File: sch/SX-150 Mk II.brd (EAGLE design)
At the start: 156.2 x 60.6 mm, 189 parts, among them IC1 LM358D, IC2 74HC02D, IC3 LM358D, IC4 LM386M-1, IC5 NJU7096, IC6 REG1117, J1 PJ301M, J2 Line In, Q1 2SC2712, Q10 2SC2712, Q11 2SA1162, Q12 2SC2712, Q13 2SC2712, Q14 2SC2712, Q15 2SC2712, Q16 2SC2712, Q17 2SC2712, Q18 2SC2712, Q19 2SC2712, Q2 2SC2712, Q20 2SC2712, Q21 2SC2712, Q22 2SC2712, Q23 2SC2712, Q24 2SA1162, Q25 2SC2712, Q26 2SC2712, Q27 2SC2712, Q28 2SC2712, Q3 2SC2712, Q4 2SC2712, Q5 2SC2712, Q6 2SC2712, Q7 2SC2712, Q8 2SA1162, Q9 2SC2712, SW1 SP3T, T1 50k, X2 Speaker Out

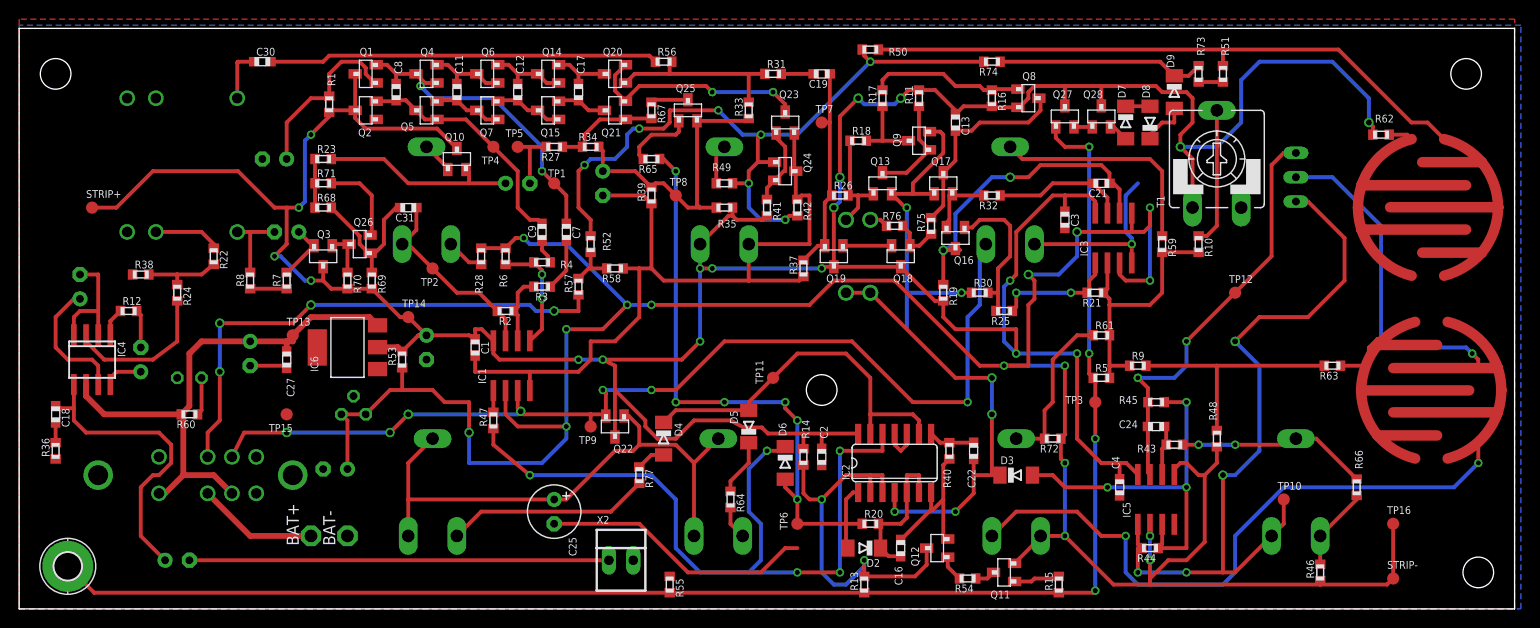
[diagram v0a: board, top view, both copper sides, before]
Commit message: Updating board layout and adding gerbers
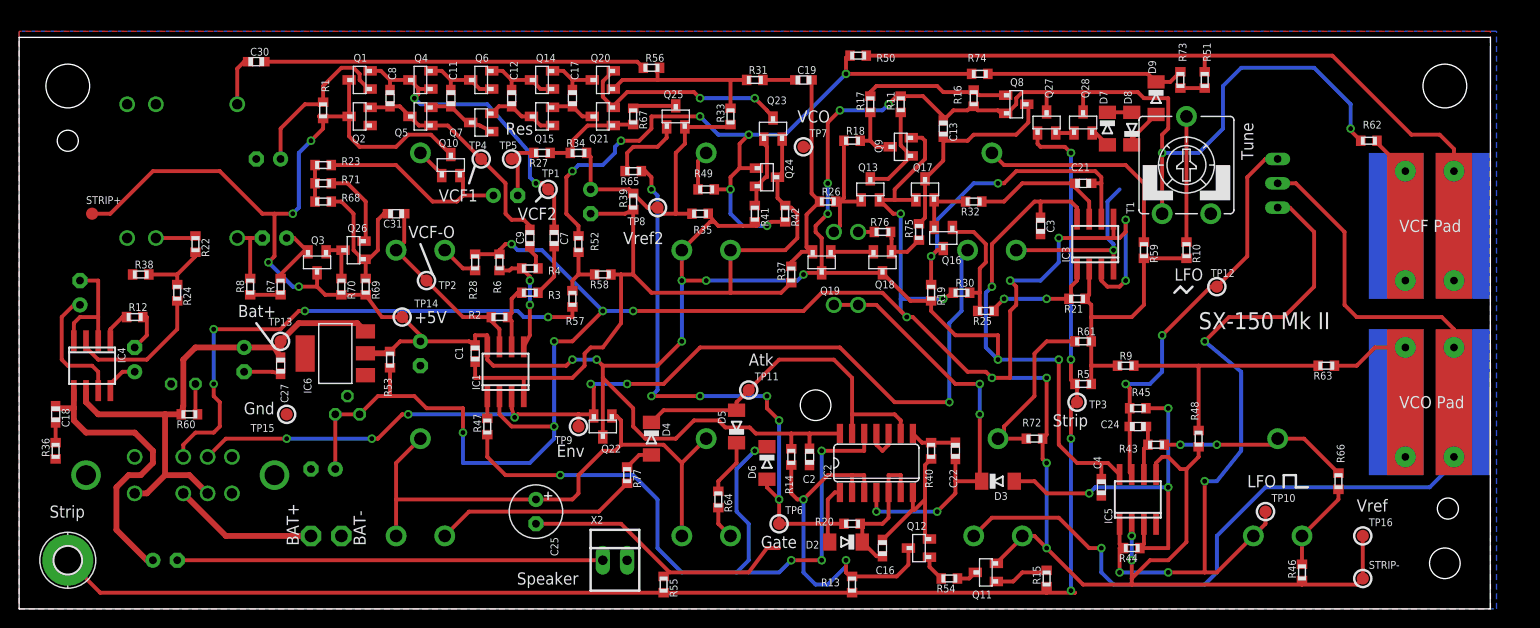
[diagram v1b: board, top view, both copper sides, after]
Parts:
- FINGERPAD2, PAD1: value FINGERPAD-2A -> GAKKEN-PAD; device dom-key:FINGERPAD-2A -> dom-key:GAKKEN-PAD
- moved TP16 3.42 mm to (140.3, 7.62)
- moved T1 3.24 mm to (121.9, 46.4)
- moved TP7 3.17 mm to (81.9, 48.3)
- moved STRIP- 3.17 mm to (140.3, 3.17)
- moved TP11 2.84 mm to (76.2, 22.9), turned to 0 degrees
- moved C3 2.62 mm to (106.7, 40.0)
- moved R35 2.62 mm to (71.1, 41.3)
- moved C23 2.29 mm to (59.7, 42.5)
- moved R22 2.29 mm to (18.4, 38.1)
- moved R65 2.29 mm to (64.1, 45.7)
- moved TP8 2.29 mm to (66.7, 41.9)
- moved TP10 2.29 mm to (130.2, 10.2)
- moved Q17 2.01 mm to (94.6, 43.8)
- moved Q27 2.01 mm to (107.3, 50.8)
- moved Q28 2.01 mm to (111.1, 50.8)
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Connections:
- net LFO: now also FINGERPAD2.A0, FINGERPAD2.A1; no longer FINGERPAD2.1
- net N$67: now also PAD1.B0, PAD1.B1; no longer PAD1.2
- net N$77: now also PAD1.A0, PAD1.A1; no longer PAD1.1
- net N$82: now also FINGERPAD2.B0, FINGERPAD2.B1; no longer FINGERPAD2.2
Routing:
- net N$67: track 64.6 -> 80.9 mm
- net AGND: track 314.3 -> 300.7 mm, vias 18 -> 19
- net N$77: track 2.54 -> 15.8 mm
- net N$82: track 6.77 -> 19.6 mm
- net LFO: track 114.1 -> 106.0 mm, vias 3 -> 1
- net GND: track 177.7 -> 173.5 mm
- net N$23: track 15.9 -> 12.6 mm
- net N$90: track 6.99 -> 4.22 mm
- net N$35: track 12.6 -> 15.2 mm
- net N$9: track 81.8 -> 79.4 mm
- net +5V: track 378.1 -> 380.2 mm
- net N$18: track 28.6 -> 30.5 mm
- net V+: track 57.4 -> 55.7 mm
- net N$32: track 7.99 -> 6.35 mm
- net N$37: track 11.6 -> 13.2 mm
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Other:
- board size 156.2 x 60.6 mm -> 153.7 x 59.7 mm
- board text added: "+5V"
- board text added: "Atk"
- board text added: "Bat+"
- board text added: "Env"
- board text added: "Gate"
- board text added: "Gnd"
- board text added: "LFO"
- board text added: "Res"
- board text added: "SX-150 Mk II"
- board text added: "Speaker"
- board text added: "Strip"
- board text added: "Tune"
- board text added: "VCF Pad"
- board text added: "VCF-O"
- board text added: "VCF1"
- board text added: "VCF2"
- board text added: "VCO"
- board text added: "VCO Pad"
- board text added: "Vref"
- board text added: "Vref2"
